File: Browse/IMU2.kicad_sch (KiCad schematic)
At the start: 6 parts, among them U2 262-BMI088

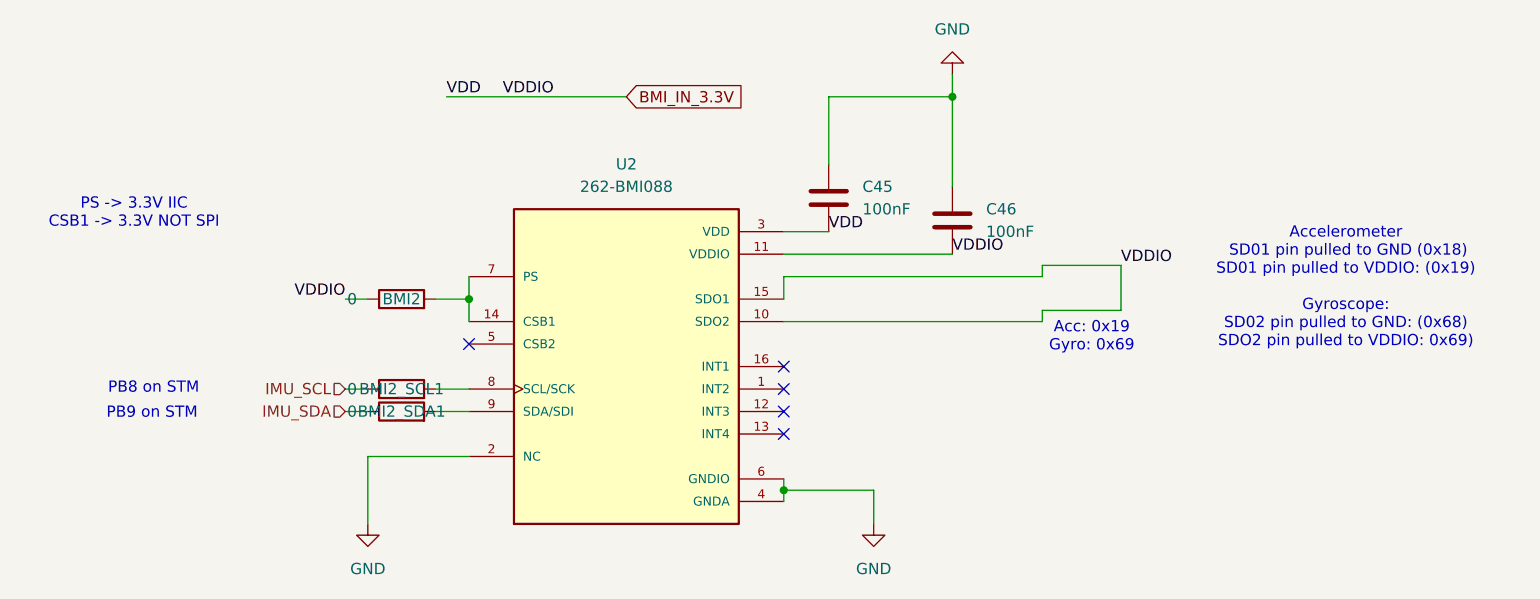
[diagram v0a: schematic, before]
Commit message: Deploying to gh-pages from @ Nautilus-UUV/nautilus-mainboard-PCB@a81f7ffbfc5f9b51f47d7f388c30fcea2673b9ea 🚀
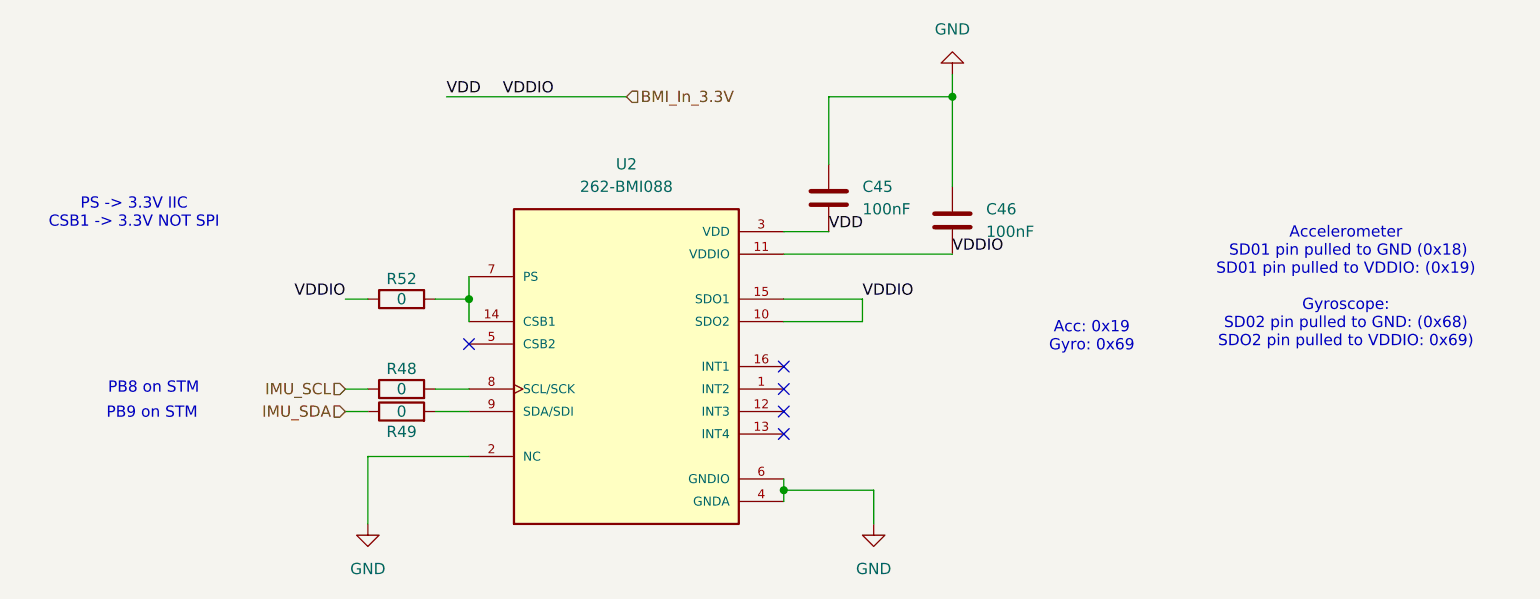
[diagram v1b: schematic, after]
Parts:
- removed BMI2, BMI2_SCL1, BMI2_SDA1: 0, Resistor_SMD:R_0603_1608Metric, symbol #dzdb:g_res/R-0-0603
- added R48, R49, R52: 0, Resistor_SMD:R_0603_1608Metric, symbol #dzdb:g_res/R-0-0603
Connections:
- net IMU_SCL: now also R48.1
- net IMU_SDA: now also R49.1
- net at U2.8 (SCL/SCK): now also R48.2
- net at U2.14 (CSB1), U2.7 (PS): now also R52.2
- net at U2.9 (SDA/SDI): now also R49.2
- net BMI_IN_3.3V renamed BMI_In_3.3V
- net BMI_In_3.3V: now also R52.1
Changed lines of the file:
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@@
-    (stroke (width 0) (type default))
-  )
-  (wire (pts (xy 191.77 90.17) (xy 200.66 90.17))
     (stroke (width 0) (type default))
   )
@@
     (stroke (width 0) (type default))
   )
-  (wire (pts (xy 200.66 90.17) (xy 200.66 85.09))
-    (stroke (width 0) (type default))
-  )
   (wire (pts (xy 172.72 110.49) (xy 172.72 114.3))
     (stroke (width 0) (type default))
@@
     (stroke (width 0) (type default))
   )
-  (wire (pts (xy 162.56 91.44) (xy 191.77 91.44))
-    (stroke (width 0) (type default))
-  )
-  (wire (pts (xy 191.77 85.09) (xy 200.66 85.09))
+  (wire (pts (xy 171.45 88.9) (xy 162.56 88.9))
+    (stroke (width 0) (type default))
+  )
+  (wire (pts (xy 162.56 91.44) (xy 171.45 91.44))
+    (stroke (width 0) (type default))
+  )
+  (wire (pts (xy 171.45 88.9) (xy 171.45 91.44))
     (stroke (width 0) (type default))
   )
@@
     (stroke (width 0) (type default))
   )
-  (wire (pts (xy 191.77 86.36) (xy 162.56 86.36))
-    (stroke (width 0) (type default))
-  )
   (wire (pts (xy 167.64 73.66) (xy 167.64 66.04))
     (stroke (width 0) (type default))
   )
-  (wire (pts (xy 162.56 86.36) (xy 162.56 88.9))
-    (stroke (width 0) (type default))
-  )
   (wire (pts (xy 113.03 99.06) (xy 115.57 99.06))
     (stroke (width 0) (type default))
@@
     (stroke (width 0) (type default))
   )
-  (wire (pts (xy 191.77 85.09) (xy 191.77 86.36))
-    (stroke (width 0) (type default))
-  )
   (wire (pts (xy 115.57 106.68) (xy 115.57 114.3))
     (stroke (width 0) (type default))
@@
   )
   (wire (pts (xy 113.03 101.6) (xy 115.57 101.6))
-    (stroke (width 0) (type default))
-  )
-  (wire (pts (xy 191.77 90.17) (xy 191.77 91.44))
     (stroke (width 0) (type default))
   )
@@
     (effects (font (size 1.27 1.27)) (justify left bottom))
   )
-  (label "VDDIO" (at 200.66 85.09 0)
+  (label "VDDIO" (at 171.45 88.9 0)
     (effects (font (size 1.27 1.27)) (justify left bottom))
   )
@@
     (effects (font (size 1.27 1.27)) (justify right bottom))
   )
-  (global_label "BMI_IN_3.3V" (shape input) (at 144.78 66.04 0) (fields_autoplaced)
-    (effects (font (size 1.27 1.27)) (justify left))
-    (property "Intersheetrefs" "${INTERSHEET_REFS}" (at 159.0743 66.04 0)
-      (effects (font (size 1.27 1.27)) (justify left) (hide yes))
-    )
-  )
   (hierarchical_label "IMU_SDA" (shape input) (at 113.03 101.6 180)
     (effects (font (size 1.27 1.27)) (justify right))
@@
   (hierarchical_label "IMU_SCL" (shape input) (at 113.03 99.06 180)
     (effects (font (size 1.27 1.27)) (justify right))
+  )
+  (hierarchical_label "BMI_In_3.3V" (shape input) (at 144.78 66.04 0)
+    (effects (font (size 1.27 1.27)) (justify left))
   )
   (symbol (lib_id "power:GND") (at 181.61 63.5 180) (unit 1)
@@
     )
   )
+  (symbol (lib_id "#dzdb:g_res/R-0-0603") (at 119.38 88.9 90) (unit 1)
+    (exclude_from_sim no) (in_bom yes) (on_board yes) (dnp no)
+    (property "Reference" "R52" (at 119.38 86.614 90)
+      (effects (font (size 1.27 1.27)))
+    )
+    (property "Value" "0" (at 119.38 88.9 90)
+      (effects (font (size 1.27 1.27)))
+    )
+    (property "Footprint" "Resistor_SMD:R_0603_1608Metric" (at 119.38 90.678 90)
+      (effects (font (size 1.27 1.27)) (hide yes))
+    )
+    (property "Datasheet" "https://www.we-online.com/components/products/datasheet/560112116001.pdf" (at 119.38 88.9 0)
+      (effects (font (size 1.27 1.27)) (hide yes))
+    )
+    (property "Description" "Thick Film Resistors - SMD WRIS-RSKS <0.05 Ohms  0.1 W Jumper 0603" (at 119.38 88.9 0)
+      (effects (font (size 1.27 1.27)) (hide yes))
+    )
+    (property "IPN" "R-0-0603" (at 119.38 88.9 0)
+      (effects (font (size 1.27 1.27)) (hide yes))
+    )
+    (property "MPN" "560112116001" (at 119.38 88.9 0)
+      (effects (font (size 1.27 1.27)) (hide yes))
+    )
+    (property "Manufacturer" "Wurth Elektronik" (at 119.38 88.9 0)
+      (effects (font (size 1.27 1.27)) (hide yes))
+    )
+    (property "Resistance" "0" (at 119.38 88.9 0)
+      (effects (font (size 1.27 1.27)) (hide yes))
+    )
+    (property "Power" "0.1W" (at 119.38 88.9 0)
+      (effects (font (size 1.27 1.27)) (hide yes))
+    )
+    (property "Material" "Thick film" (at 119.38 88.9 0)
+      (effects (font (size 1.27 1.27)) (hide yes))
+    )
+    (property "Tolerance" "5%" (at 119.38 88.9 0)
+      (effects (font (size 1.27 1.27)) (hide yes))
+    )
+    (property "Supplier" "Mouser" (at 119.38 88.9 0)
+      (effects (font (size 1.27 1.27)) (hide yes))
+    )
+    (property "SPN" "710-560112116001" (at 119.38 88.9 0)
+      (effects (font (size 1.27 1.27)) (hide yes))
+    )
+    (property "LCSC" "CXXXXX" (at 119.38 88.9 0)
+      (effects (font (size 1.27 1.27)) (hide yes))
+    )
+    (property "Comment" "lifecycle=Active; note=Auto-generated" (at 119.38 88.9 0)
+      (effects (font (size 1.27 1.27)) (hide yes))
+    )
+    (pin "1")
+    (pin "2")
+    (instances
+      (project "nautilus_mainboard"
+        (path "/ce1819b2-f280-40ed-834f-6fe4d12f809d/bdf8f7d6-a5ee-4741-925d-5019e8cbdfce/a7ffb13a-d9ae-4b81-b70f-0aefcfc6ef00"
+          (reference "R52") (unit 1)
+        )
+      )
+    )
+  )
   (symbol (lib_id "power:GND") (at 115.57 114.3 0) (unit 1)
     (exclude_from_sim no) (in_bom yes) (on_board yes) (dnp no) (fields_autoplaced)
@@
   (symbol (lib_id "#dzdb:g_res/R-0-0603") (at 119.38 99.06 90) (unit 1)
     (exclude_from_sim no) (in_bom yes) (on_board yes) (dnp no)
-    (property "Reference" "BMI2_SCL1" (at 119.38 99.06 90)
-      (effects (font (size 1.27 1.27)))
-    )
-    (property "Value" "0" (at 113.792 99.06 90)
+    (property "Reference" "R48" (at 119.38 96.774 90)
+      (effects (font (size 1.27 1.27)))
+    )
+    (property "Value" "0" (at 119.38 99.06 90)
       (effects (font (size 1.27 1.27)))
     )
@@
       (effects (font (size 1.27 1.27)) (hide yes))
     )
+    (pin "1")
     (pin "2")
-    (pin "1")
-    (instances
-      (project "nautilus_mainboard"
-        (path "/ce1819b2-f280-40ed-834f-6fe4d12f809d/bdf8f7d6-a5ee-4741-925d-5019e8cbdfce/a7ffb13a-d9ae-4b81-b70f-0aefcfc6ef00"
-          (reference "BMI2_SCL1") (unit 1)
+    (instances
+      (project "nautilus_mainboard"
+        (path "/ce1819b2-f280-40ed-834f-6fe4d12f809d/bdf8f7d6-a5ee-4741-925d-5019e8cbdfce/a7ffb13a-d9ae-4b81-b70f-0aefcfc6ef00"
+          (reference "R48") (unit 1)
         )
       )
@@
     )
   )
-  (symbol (lib_id "#dzdb:g_res/R-0-0603") (at 119.38 88.9 90) (unit 1)
-    (exclude_from_sim no) (in_bom yes) (on_board yes) (dnp no)
-    (property "Reference" "BMI2" (at 119.38 88.9 90)
-      (effects (font (size 1.27 1.27)))
-    )
-    (property "Value" "0" (at 113.792 88.9 90)
-      (effects (font (size 1.27 1.27)))
-    )
-    (property "Footprint" "Resistor_SMD:R_0603_1608Metric" (at 119.38 90.678 90)
-      (effects (font (size 1.27 1.27)) (hide yes))
-    )
-    (property "Datasheet" "https://www.we-online.com/components/products/datasheet/560112116001.pdf" (at 119.38 88.9 0)
-      (effects (font (size 1.27 1.27)) (hide yes))
-    )
-    (property "Description" "Thick Film Resistors - SMD WRIS-RSKS <0.05 Ohms  0.1 W Jumper 0603" (at 119.38 88.9 0)
-      (effects (font (size 1.27 1.27)) (hide yes))
-    )
-    (property "IPN" "R-0-0603" (at 119.38 88.9 0)
-      (effects (font (size 1.27 1.27)) (hide yes))
-    )
-    (property "MPN" "560112116001" (at 119.38 88.9 0)
-      (effects (font (size 1.27 1.27)) (hide yes))
-    )
-    (property "Manufacturer" "Wurth Elektronik" (at 119.38 88.9 0)
-      (effects (font (size 1.27 1.27)) (hide yes))
-    )
-    (property "Resistance" "0" (at 119.38 88.9 0)
-      (effects (font (size 1.27 1.27)) (hide yes))
-    )
-    (property "Power" "0.1W" (at 119.38 88.9 0)
-      (effects (font (size 1.27 1.27)) (hide yes))
-    )
-    (property "Material" "Thick film" (at 119.38 88.9 0)
-      (effects (font (size 1.27 1.27)) (hide yes))
-    )
-    (property "Tolerance" "5%" (at 119.38 88.9 0)
-      (effects (font (size 1.27 1.27)) (hide yes))
-    )
-    (property "Supplier" "Mouser" (at 119.38 88.9 0)
-      (effects (font (size 1.27 1.27)) (hide yes))
-    )
-    (property "SPN" "710-560112116001" (at 119.38 88.9 0)
-      (effects (font (size 1.27 1.27)) (hide yes))
-    )
-    (property "LCSC" "CXXXXX" (at 119.38 88.9 0)
-      (effects (font (size 1.27 1.27)) (hide yes))
-    )
-    (property "Comment" "lifecycle=Active; note=Auto-generated" (at 119.38 88.9 0)
-      (effects (font (size 1.27 1.27)) (hide yes))
-    )
-    (pin "2")
-    (pin "1")
-    (instances
-      (project "nautilus_mainboard"
-        (path "/ce1819b2-f280-40ed-834f-6fe4d12f809d/bdf8f7d6-a5ee-4741-925d-5019e8cbdfce/a7ffb13a-d9ae-4b81-b70f-0aefcfc6ef00"
-          (reference "BMI2") (unit 1)
-        )
-      )
-    )
-  )
   (symbol (lib_id "#dzdb:g_cap/C-100n-0603") (at 167.64 77.47 0) (unit 1)
     (exclude_from_sim no) (in_bom yes) (on_board yes) (dnp no) (fields_autoplaced)
@@
   (symbol (lib_id "#dzdb:g_res/R-0-0603") (at 119.38 101.6 90) (unit 1)
     (exclude_from_sim no) (in_bom yes) (on_board yes) (dnp no)
-    (property "Reference" "BMI2_SDA1" (at 119.38 101.6 90)
-      (effects (font (size 1.27 1.27)))
-    )
-    (property "Value" "0" (at 113.792 101.6 90)
+    (property "Reference" "R49" (at 119.38 103.886 90)
+      (effects (font (size 1.27 1.27)))
+    )
+    (property "Value" "0" (at 119.38 101.6 90)
       (effects (font (size 1.27 1.27)))
     )
@@
       (effects (font (size 1.27 1.27)) (hide yes))
     )
+    (pin "1")
     (pin "2")
-    (pin "1")
-    (instances
-      (project "nautilus_mainboard"
-        (path "/ce1819b2-f280-40ed-834f-6fe4d12f809d/bdf8f7d6-a5ee-4741-925d-5019e8cbdfce/a7ffb13a-d9ae-4b81-b70f-0aefcfc6ef00"
-          (reference "BMI2_SDA1") (unit 1)
-        )
-      )
+    (instances
+      (project "nautilus_mainboard"
+        (path "/ce1819b2-f280-40ed-834f-6fe4d12f809d/bdf8f7d6-a5ee-4741-925d-5019e8cbdfce/a7ffb13a-d9ae-4b81-b70f-0aefcfc6ef00"
+          (reference "R49") (unit 1)
+        )
+      )
